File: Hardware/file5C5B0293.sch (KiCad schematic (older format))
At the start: 27 parts, among them J16 Conn_01x06_Male, J17 Conn_ARM_JTAG_SWD_10, J24 Digital_Connector, J25 CV_Connector, J26 Pot_Connector, J27 Attenuverter_Connector, U13 STM32F303RBTx

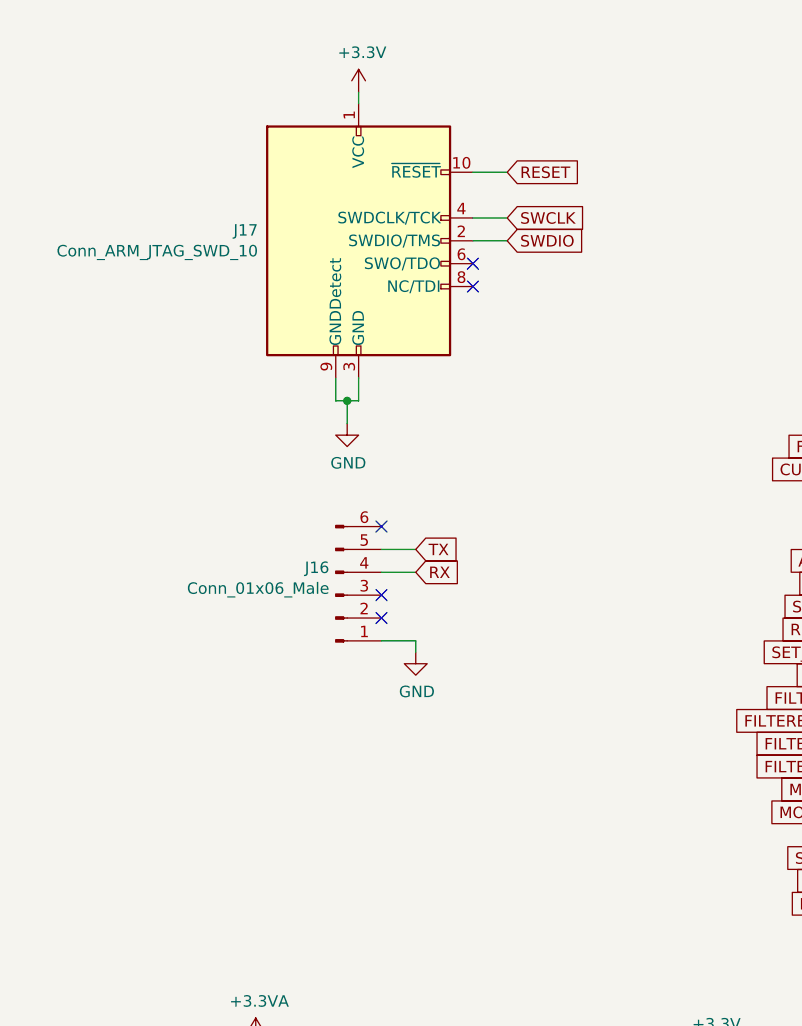
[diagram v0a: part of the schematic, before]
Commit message: IT WORKS
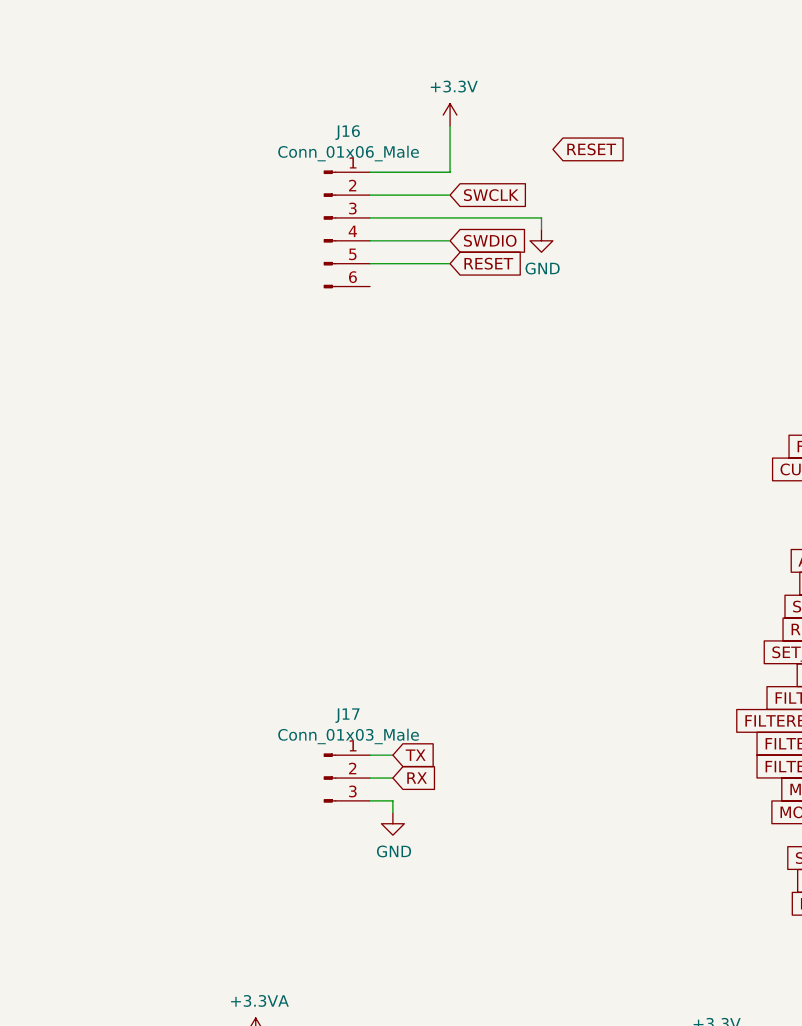
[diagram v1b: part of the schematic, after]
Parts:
- removed J17: Conn_ARM_JTAG_SWD_10, Connector_PinHeader_2.54mm:PinHeader_2x05_P2.54mm_Vertical, symbol Connector:Conn_ARM_JTAG_SWD_10
- added J17: Conn_01x03_Male, Connector_PinHeader_2.54mm:PinHeader_1x03_P2.54mm_Vertical, symbol Connector:Conn_01x03_Male
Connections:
- net +3V3: now also J16.1 (Pin_1)
- net GND: now also J16.3 (Pin_3), J17.3 (Pin_3); no longer J16.1 (Pin_1)
- net RESET: now also J16.5 (Pin_5)
- net RX: now also J17.2 (Pin_2); no longer J16.4 (Pin_4)
- net SWCLK: now also J16.2 (Pin_2)
- net SWDIO: now also J16.4 (Pin_4)
- net TX: now also J17.1 (Pin_1); no longer J16.5 (Pin_5)
- no-connect marks 16 -> 11
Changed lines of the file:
@@
 Wire Wire Line
 	1500 5750 1500 5800
-$Comp
-L power:GND #PWR0137
-U 1 1 5BF2206A
-P 1900 3050
-F 0 "#PWR0137" H 1900 2800 50  0001 C CNN
-F 1 "GND" H 1905 2877 50  0000 C CNN
-F 2 "" H 1900 3050 50  0001 C CNN
-F 3 "" H 1900 3050 50  0001 C CNN
-	1    1900 3050
-	1    0    0    -1
-$EndComp
 Wire Wire Line
 	1500 5800 1250 5800
@@
 	5250 7450 5550 7450
 $Comp
-L Connector:Conn_ARM_JTAG_SWD_10 J17
-U 1 1 5BF86C4D
-P 1950 2250
-F 0 "J17" H 1510 2296 50  0000 R CNN
-F 1 "Conn_ARM_JTAG_SWD_10" H 1510 2205 50  0000 R CNN
-F 2 "Connector_PinHeader_2.54mm:PinHeader_2x05_P2.54mm_Vertical" H 2000 1700 50  0001 L TNN
-F 3 "http://infocenter.arm.com/help/topic/com.arm.doc.faqs/attached/13634/cortex_debug_connectors.pdf" V 1600 1000 50  0001 C CNN
-	1    1950 2250
-	1    0    0    -1
-$EndComp
-Wire Wire Line
-	1900 3050 1900 2950
-Wire Wire Line
-	1900 2950 1850 2950
-Wire Wire Line
-	1850 2950 1850 2850
-Wire Wire Line
-	1950 2850 1950 2950
-Wire Wire Line
-	1950 2950 1900 2950
-Connection ~ 1900 2950
-$Comp
 L power:+3.3V #PWR0138
 U 1 1 5BF90955
-P 1950 1600
-F 0 "#PWR0138" H 1950 1450 50  0001 C CNN
-F 1 "+3.3V" H 1965 1773 50  0000 C CNN
-F 2 "" H 1950 1600 50  0001 C CNN
-F 3 "" H 1950 1600 50  0001 C CNN
-	1    1950 1600
-	1    0    0    -1
-$EndComp
-Wire Wire Line
-	1950 1600 1950 1650
-Text GLabel 2600 1950 2    50   Input ~ 0
+P 2350 1750
+F 0 "#PWR0138" H 2350 1600 50  0001 C CNN
+F 1 "+3.3V" H 2365 1923 50  0000 C CNN
+F 2 "" H 2350 1750 50  0001 C CNN
+F 3 "" H 2350 1750 50  0001 C CNN
+	1    2350 1750
+	1    0    0    -1
+$EndComp
+Text GLabel 2800 1850 2    50   Input ~ 0
 RESET
-Wire Wire Line
-	2600 1950 2450 1950
 Text GLabel 6500 3150 2    50   Input ~ 0
 SET_SW
 Text GLabel 6500 3350 2    50   Input ~ 0
 SWCLK
-Text GLabel 2600 2250 2    50   Input ~ 0
+Text GLabel 2350 2250 2    50   Input ~ 0
 SWDIO
-Wire Wire Line
-	2600 2250 2450 2250
-Text GLabel 2600 2150 2    50   Input ~ 0
+Text GLabel 2350 2050 2    50   Input ~ 0
 SWCLK
-Wire Wire Line
-	2600 2150 2450 2150
-$Comp
-L Connector:Conn_01x06_Male J16
-U 1 1 5BFB55EB
-P 1850 3800
-F 0 "J16" H 1822 3680 50  0000 R CNN
-F 1 "Conn_01x06_Male" H 1822 3771 50  0000 R CNN
-F 2 "Connector_PinHeader_2.54mm:PinHeader_1x06_P2.54mm_Vertical" H 1850 3800 50  0001 C CNN
-F 3 "~" H 1850 3800 50  0001 C CNN
-	1    1850 3800
-	1    0    0    1
-$EndComp
 Text GLabel 6500 2850 2    50   Input ~ 0
 TX
 Text GLabel 6500 2950 2    50   Input ~ 0
 RX
-Text GLabel 2200 3600 2    50   Input ~ 0
+Text GLabel 2100 4500 2    50   Input ~ 0
 TX
-Wire Wire Line
-	2200 3600 2050 3600
-Text GLabel 2200 3700 2    50   Input ~ 0
+Text GLabel 2100 4600 2    50   Input ~ 0
 RX
-Wire Wire Line
-	2200 3700 2050 3700
 $Comp
 L power:GND #PWR0139
 U 1 1 5BFD1A9D
-P 2200 4050
-F 0 "#PWR0139" H 2200 3800 50  0001 C CNN
-F 1 "GND" H 2205 3877 50  0000 C CNN
-F 2 "" H 2200 4050 50  0001 C CNN
-F 3 "" H 2200 4050 50  0001 C CNN
-	1    2200 4050
-	1    0    0    -1
-$EndComp
-Wire Wire Line
-	2200 4050 2200 4000
-Wire Wire Line
-	2200 4000 2050 4000
-NoConn ~ 2050 3500
-NoConn ~ 2050 3800
-NoConn ~ 2050 3900
-NoConn ~ 2450 2350
-NoConn ~ 2450 2450
+P 2100 4750
+F 0 "#PWR0139" H 2100 4500 50  0001 C CNN
+F 1 "GND" H 2105 4577 50  0000 C CNN
+F 2 "" H 2100 4750 50  0001 C CNN
+F 3 "" H 2100 4750 50  0001 C CNN
+	1    2100 4750
+	1    0    0    -1
+$EndComp
 Text GLabel 4200 4050 0    50   Input ~ 0
 SET_ATTEN
@@
 NoConn ~ 9900 2650
 NoConn ~ 9900 2750
+$Comp
+L Connector:Conn_01x03_Male J17
+U 1 1 5C9CB1BC
+P 1800 4600
+F 0 "J17" H 1906 4878 50  0000 C CNN
+F 1 "Conn_01x03_Male" H 1906 4787 50  0000 C CNN
+F 2 "Connector_PinHeader_2.54mm:PinHeader_1x03_P2.54mm_Vertical" H 1800 4600 50  0001 C CNN
+F 3 "~" H 1800 4600 50  0001 C CNN
+	1    1800 4600
+	1    0    0    -1
+$EndComp
+Wire Wire Line
+	2100 4750 2100 4700
+Wire Wire Line
+	2100 4700 2000 4700
+Wire Wire Line
+	2100 4600 2000 4600
+Wire Wire Line
+	2100 4500 2000 4500
+$Comp
+L Connector:Conn_01x06_Male J16
+U 1 1 5CA02872
+P 1800 2150
+F 0 "J16" H 1906 2528 50  0000 C CNN
+F 1 "Conn_01x06_Male" H 1906 2437 50  0000 C CNN
+F 2 "Connector_PinHeader_2.54mm:PinHeader_1x06_P2.54mm_Vertical" H 1800 2150 50  0001 C CNN
+F 3 "~" H 1800 2150 50  0001 C CNN
+	1    1800 2150
+	1    0    0    -1
+$EndComp
+Wire Wire Line
+	2000 1950 2350 1950
+Wire Wire Line
+	2350 1950 2350 1750
+Wire Wire Line
+	2350 2050 2000 2050
+$Comp
+L power:GND #PWR0163
+U 1 1 5CA355D8
+P 2750 2200
+F 0 "#PWR0163" H 2750 1950 50  0001 C CNN
+F 1 "GND" H 2755 2027 50  0000 C CNN
+F 2 "" H 2750 2200 50  0001 C CNN
+F 3 "" H 2750 2200 50  0001 C CNN
+	1    2750 2200
+	1    0    0    -1
+$EndComp
+Wire Wire Line
+	2750 2200 2750 2150
+Wire Wire Line
+	2750 2150 2000 2150
+Wire Wire Line
+	2350 2250 2000 2250
+Text GLabel 2350 2350 2    50   Input ~ 0
+RESET
+Wire Wire Line
+	2350 2350 2000 2350
 $EndSCHEMATC
